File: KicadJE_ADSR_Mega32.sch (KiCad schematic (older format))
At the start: 41 parts, among them J101 ADSR1, J102 ADSR2, J105 ADSR1-G8, J106 ADSR2-G8, J107 ADSR4-G8, J108 ADSR3-G8

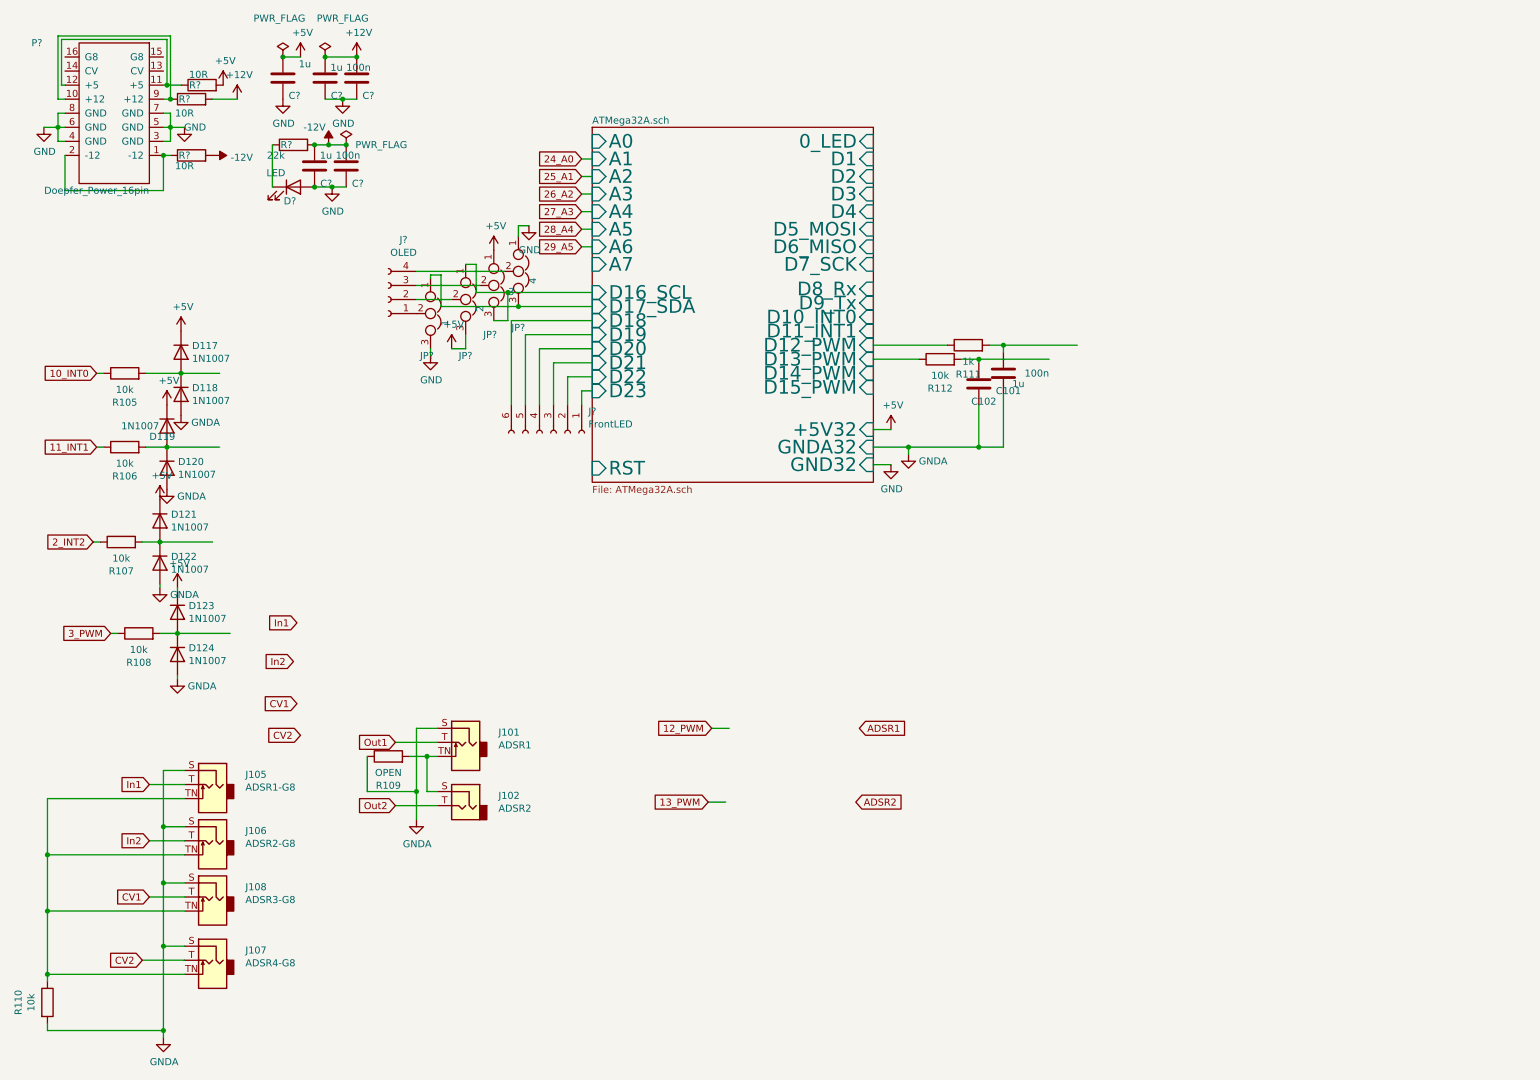
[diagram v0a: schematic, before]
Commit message: Cleanup MasterSCH
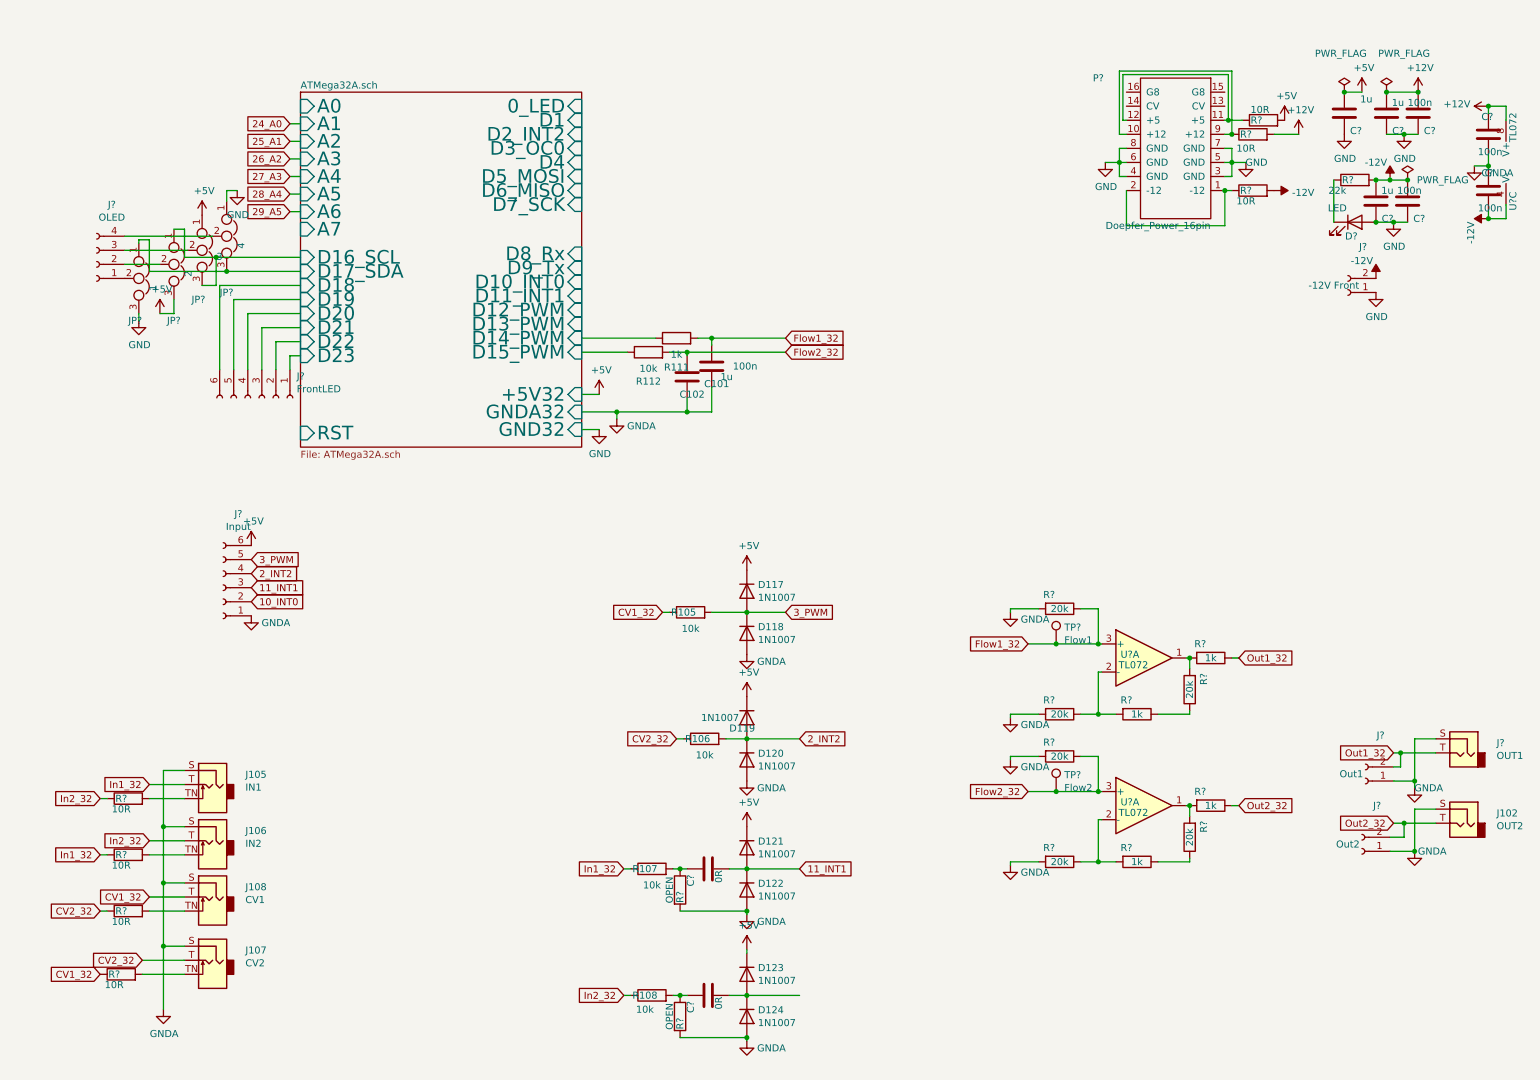
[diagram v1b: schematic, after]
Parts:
- removed J101: ADSR1, AJ-Dropbox-Kicad:PJ301SM, symbol Connector:AudioJack2_SwitchT
- removed R109: OPEN, Resistor_SMD:R_0805_2012Metric_Pad1.15x1.40mm_HandSolder, symbol Device:R
- removed R110: 10k, Resistor_SMD:R_0805_2012Metric_Pad1.15x1.40mm_HandSolder, symbol Device:R
- added C? (x2): 100n, AJ:C_0805_AJ, symbol Device:C
- added C? (x2): 0R, AJ:C_0805_AJ, symbol Device:C
- added J?: OUT1, AJ-Dropbox-Kicad:PJ301SM, symbol Connector:AudioJack2
- added J?: Input, Connector_PinSocket_2.54mm:PinSocket_1x06_P2.54mm_Vertical, symbol Connector:Conn_01x06_Female
- added J?: Out1, Connector_PinSocket_2.54mm:PinSocket_1x02_P2.54mm_Vertical, symbol Connector:Conn_01x02_Female
- added J?: Out2, Connector_PinSocket_2.54mm:PinSocket_1x02_P2.54mm_Vertical, symbol Connector:Conn_01x02_Female
- added J?: -12V Front, Connector_PinSocket_2.54mm:PinSocket_1x02_P2.54mm_Vertical, symbol Connector:Conn_01x02_Female
- added R? (x4): 1k, Resistor_SMD:R_0805_2012Metric_Pad1.15x1.40mm_HandSolder, symbol Device:R
- added R? (x6): 20k, Resistor_SMD:R_0805_2012Metric_Pad1.15x1.40mm_HandSolder, symbol Device:R
- added R? (x4): 10R, Resistor_SMD:R_0805_2012Metric_Pad1.15x1.40mm_HandSolder, symbol Device:R
- added R? (x2): OPEN, Resistor_SMD:R_0805_2012Metric_Pad1.15x1.40mm_HandSolder, symbol Device:R
- added TP?: Flow1, TestPoint:TestPoint_THTPad_2.0x2.0mm_Drill1.0mm, symbol Connector:TestPoint
- added TP?: Flow2, TestPoint:TestPoint_THTPad_2.0x2.0mm_Drill1.0mm, symbol Connector:TestPoint
- added U? (x3): TL072, AJ-Dropbox-Kicad:AJ_SO-8_5.3x6.2mm_P1.27mm, symbol Amplifier_Operational:TL072
- C101, C102: footprint Capacitor_SMD:C_0805_2012Metric_Pad1.15x1.40mm_HandSolder -> Capacitor_SMD:C_1206_3216Metric
- C? (x2): footprint Capacitor_SMD:C_0805_2012Metric_Pad1.15x1.40mm_HandSolder -> AJ:C_0805_AJ
- C? (x3): footprint Capacitor_SMD:C_1206_3216Metric_Pad1.42x1.75mm_HandSolder -> AJ:C_0805_AJ
- J102: value ADSR2 -> OUT2
- J105: value ADSR1-G8 -> IN1
- J106: value ADSR2-G8 -> IN2
- J107: value ADSR4-G8 -> CV2
- J108: value ADSR3-G8 -> CV1
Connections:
- net labels added: CV1_32, CV2_32, Flow1_32, Flow2_32, In1_32, In2_32, Out1_32, Out2_32
- net labels removed: 12_PWM, 13_PWM, ADSR1, ADSR2, CV1, CV2, In1, In2, Out1, Out2
- wire segments 141 -> 190
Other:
- moved on the sheet: C101, C102, C?, D117, D118, D119, D120, D121, D122, D123, D124, D?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
